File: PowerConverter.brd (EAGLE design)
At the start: 50 x 40 mm, 13 parts

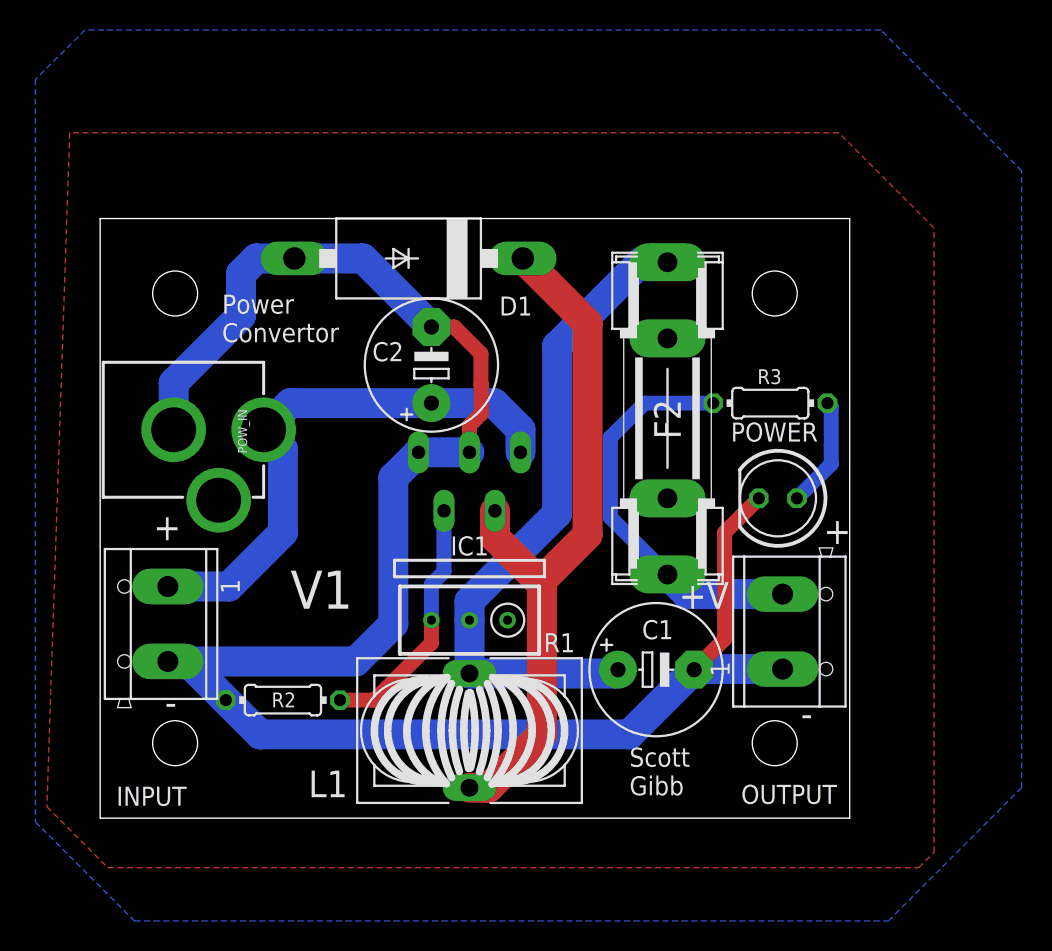
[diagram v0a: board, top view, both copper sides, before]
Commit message: Adding updated Files
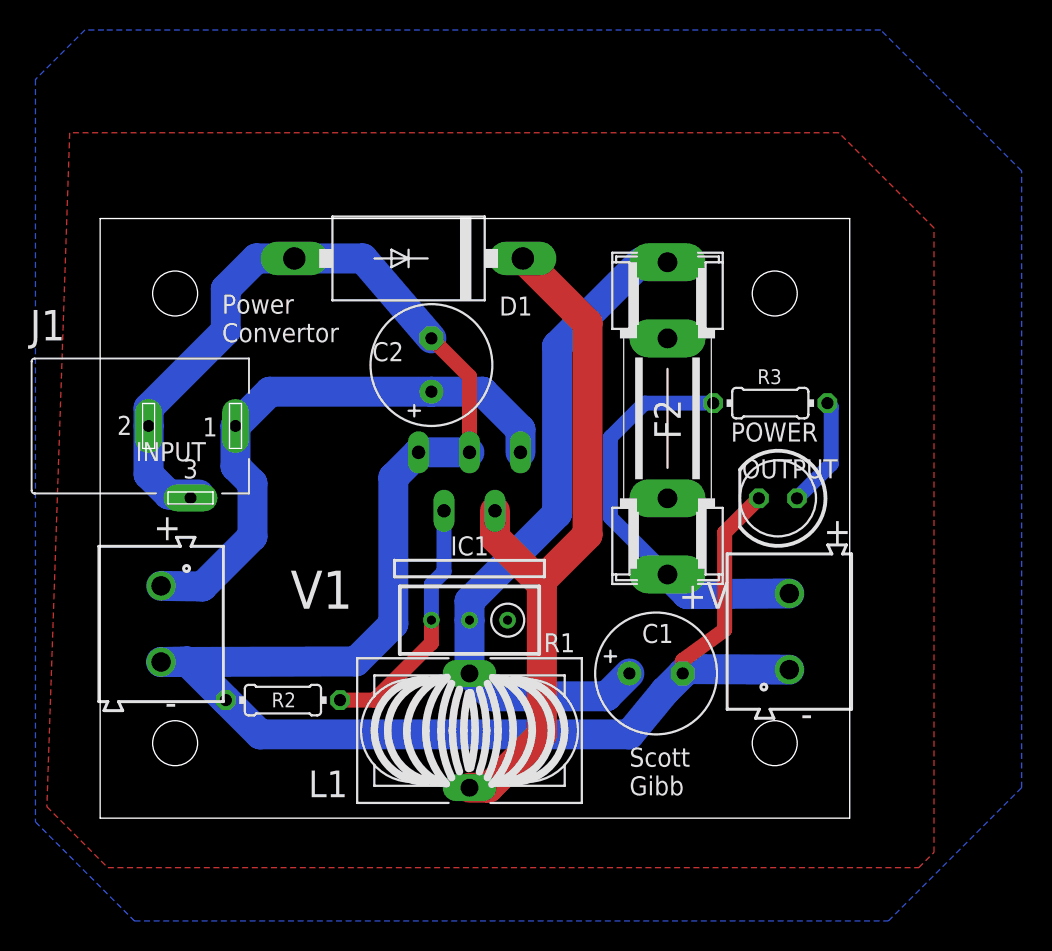
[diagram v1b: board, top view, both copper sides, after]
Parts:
- removed POW_IN: POWER_JACK, SparkFun-Connectors:POWER_JACK_PTH
- added J1: 694106301002, DC Power Jacks:694106301002
- C1, C2: device rcl:E5-8,5 -> rcl:E3,5-8
- D1: device diode-1:C2673 -> diode:DO201-15
- INPUT, OUTPUT: value CON_TERMINAL_BLOCK_02-5MM -> (none); device dp_devices:TERMINAL_BLOCK_2P_5 -> Wurth_Connectors_WR-TBL Rising Cage Clamp:691213510002
- moved C1 0.25 mm to (37.1, 9.65)
- turned INPUT to 270 degrees
- turned OUTPUT to 90 degrees
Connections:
- net GND: now also J1.2, J1.3; no longer POW_IN.GND
- net VSS: now also J1.1; no longer POW_IN.PWR
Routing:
- net GND: track 127.9 -> 136.1 mm
- net VCC: track 44.0 -> 45.9 mm
- net VSS: track 36.7 -> 37.8 mm
